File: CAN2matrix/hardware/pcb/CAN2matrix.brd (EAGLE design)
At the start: 100 x 80 mm, 33 parts, among them IC1 MEGA8-P, IC2 MCP2515-E/P, IC3 MCP2515-E/P, U1 MCP2551P, U2 MCP2551P, X1 CAN1, X2 CAN2

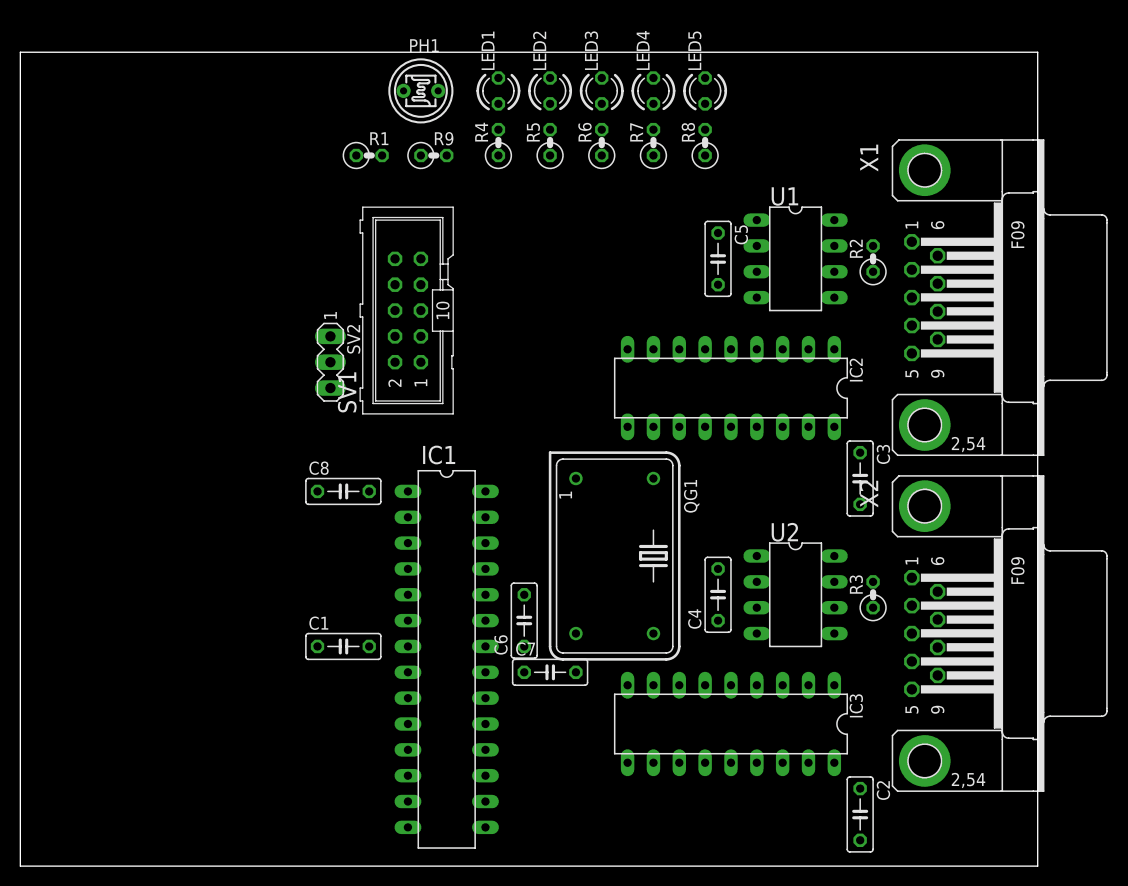
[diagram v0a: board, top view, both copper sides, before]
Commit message: V1.0 of PCB and adjusted schematics
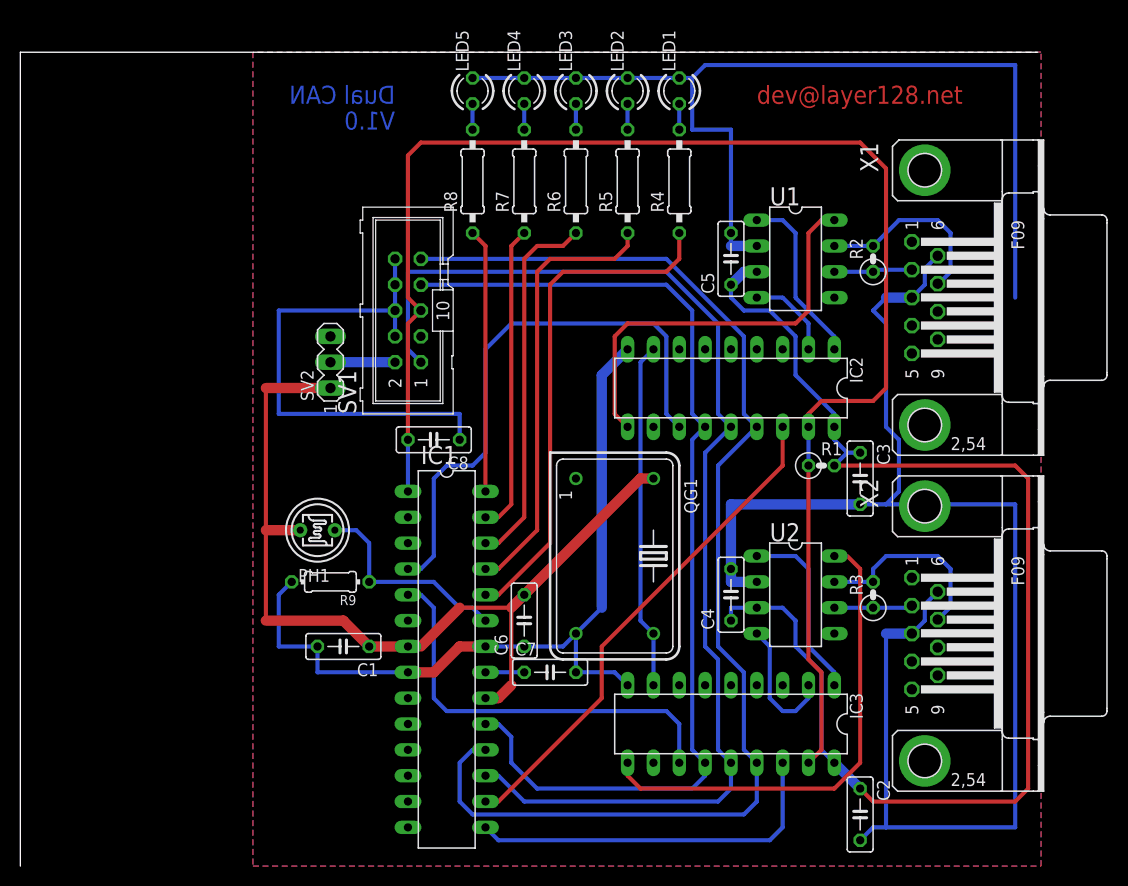
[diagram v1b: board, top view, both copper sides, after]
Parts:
- R4, R5, R6, R7, R8: device resistor:0207/2V -> resistor:0207/10
- R9: device resistor:0207/2V -> resistor:0204/7
- moved R1 53.9 mm to (78.7, 39.4)
- moved PH1 44.4 mm to (29.2, 33.0), turned to 0 degrees
- moved R9 43.1 mm to (30.5, 27.9), turned to 180 degrees
- moved R8 23.2 mm to (44.5, 67.3)
- moved LED5 22.9 mm to (44.5, 76.2)
- moved R4 18.2 mm to (64.8, 67.3)
- moved LED1 17.8 mm to (64.8, 76.2)
- moved R7 13.3 mm to (49.5, 67.3)
- moved LED4 12.7 mm to (49.5, 76.2)
- moved C8 10.2 mm to (40.6, 41.9), turned to 180 degrees
- moved R5 8.52 mm to (59.7, 67.3)
- moved LED2 7.62 mm to (59.7, 76.2)
- moved R6 4.58 mm to (54.6, 67.3)
- moved LED3 2.54 mm to (54.6, 76.2)
- moved C4 1.27 mm to (69.8, 26.7)
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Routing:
- net GND: track 0.00 -> 371.3 mm
- net +5V: track 0.00 -> 213.0 mm
- net N$9: track 0.00 -> 148.2 mm
- net N$1: track 0.00 -> 121.4 mm
- net N$2: track 0.00 -> 116.1 mm
- net N$3: track 0.00 -> 101.3 mm
- net N$16: track 0.00 -> 55.8 mm
- net N$22: track 0.00 -> 50.1 mm
- net N$14: track 0.00 -> 49.7 mm
- net N$7: track 0.00 -> 46.6 mm
- net N$23: track 0.00 -> 43.3 mm
- net N$17: track 0.00 -> 40.9 mm
- net N$19: track 0.00 -> 40.2 mm
- net N$15: track 0.00 -> 36.6 mm
- net N$24: track 0.00 -> 36.4 mm
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- added copper zone on layer 1, net +5V
- added copper zone on layer 16, net GND
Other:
- outline, holes or cut-outs redrawn
- board text added: "Dual CAN"
- board text added: "V1.0"
- board text added: "dev@layer128.net"
